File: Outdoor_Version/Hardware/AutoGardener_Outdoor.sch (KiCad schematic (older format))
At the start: 28 parts, among them J1 SWO, J2 Header_1x3, J3 Header_1x3, J4 Header_1x2, Q1 2N7002P.215, Q2 2N7002P.215, U1 STM32L031K6T6, U2 AP2204RB-3.3TRG1

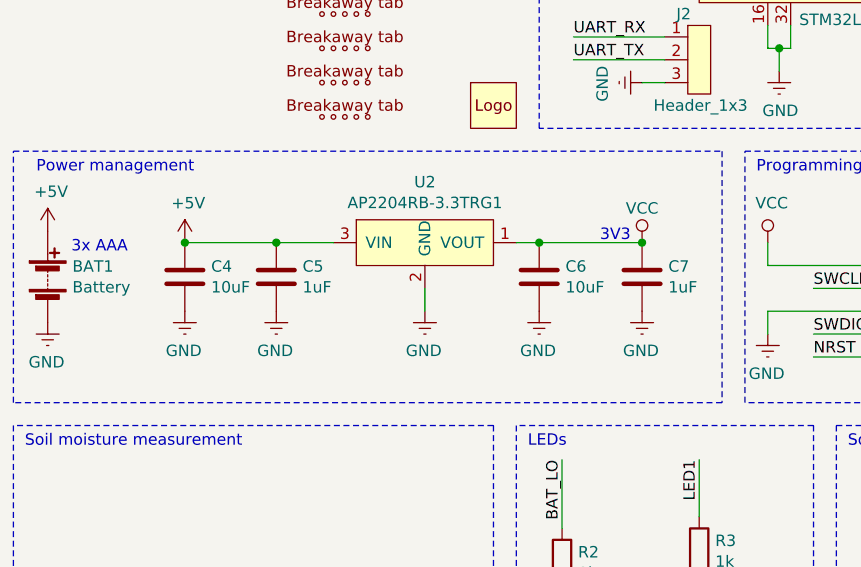
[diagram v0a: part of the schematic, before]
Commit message: Merging.
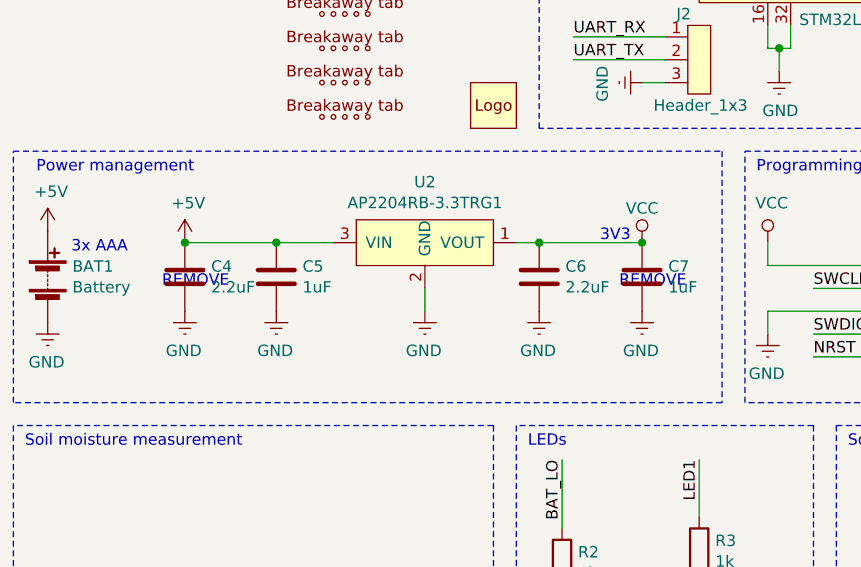
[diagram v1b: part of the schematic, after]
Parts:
- C4, C6: value 10uF -> 2.2uF; TME CL10A106MO8NQNC -> CL10A225KP8NNNC
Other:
- note added: "REMOVE"
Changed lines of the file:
@@
 P 6800 4250
 F 0 "C4" H 6915 4296 50  0000 L CNN
-F 1 "10uF" H 6915 4205 50  0000 L CNN
+F 1 "2.2uF" H 6915 4205 50  0000 L CNN
 F 2 "MRS_Passives:C0603" H 6800 3750 50  0001 C CNN
 F 3 "" H 6825 4350 50  0001 C CNN
-F 4 "CL10A106MO8NQNC" H 6800 4250 50  0001 C CNN "TME"
+F 4 "CL10A225KP8NNNC" H 6800 4250 50  0001 C CNN "TME"
 	1    6800 4250
 	1    0    0    -1
@@
 P 8350 4250
 F 0 "C6" H 8465 4296 50  0000 L CNN
-F 1 "10uF" H 8465 4205 50  0000 L CNN
+F 1 "2.2uF" H 8465 4205 50  0000 L CNN
 F 2 "MRS_Passives:C0603" H 8350 3750 50  0001 C CNN
 F 3 "" H 8375 4350 50  0001 C CNN
-F 4 "CL10A106MO8NQNC" H 8350 4250 50  0001 C CNN "TME"
+F 4 "CL10A225KP8NNNC" H 8350 4250 50  0001 C CNN "TME"
 	1    8350 4250
 	1    0    0    -1
@@
 	1    0    0    -1
 $EndComp
+Text Notes 6700 4300 0    50   ~ 0
+REMOVE
+Text Notes 8700 4300 0    50   ~ 0
+REMOVE
 $EndSCHEMATC
